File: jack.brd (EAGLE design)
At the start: 44.2 x 26.4 mm, 35 parts, among them IC1 NUF2221W1T2G, IC2 ATSAMD21G18, IC3 LDO, J1 USB-micro, SW1 SPST3.5X6MM, X1 CX-3225 12.288MHz

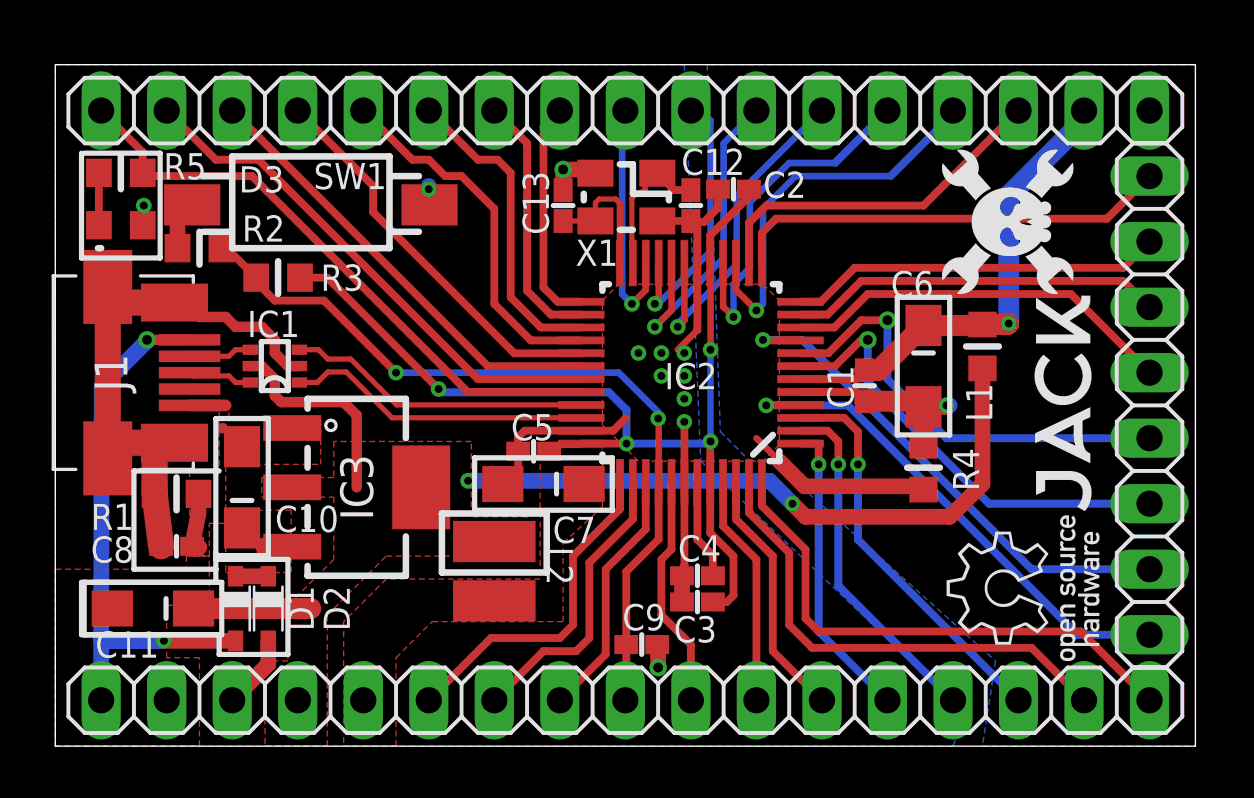
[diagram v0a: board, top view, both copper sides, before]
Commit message: :feelsgood: Added BOM, Gerbers, 3D model and render
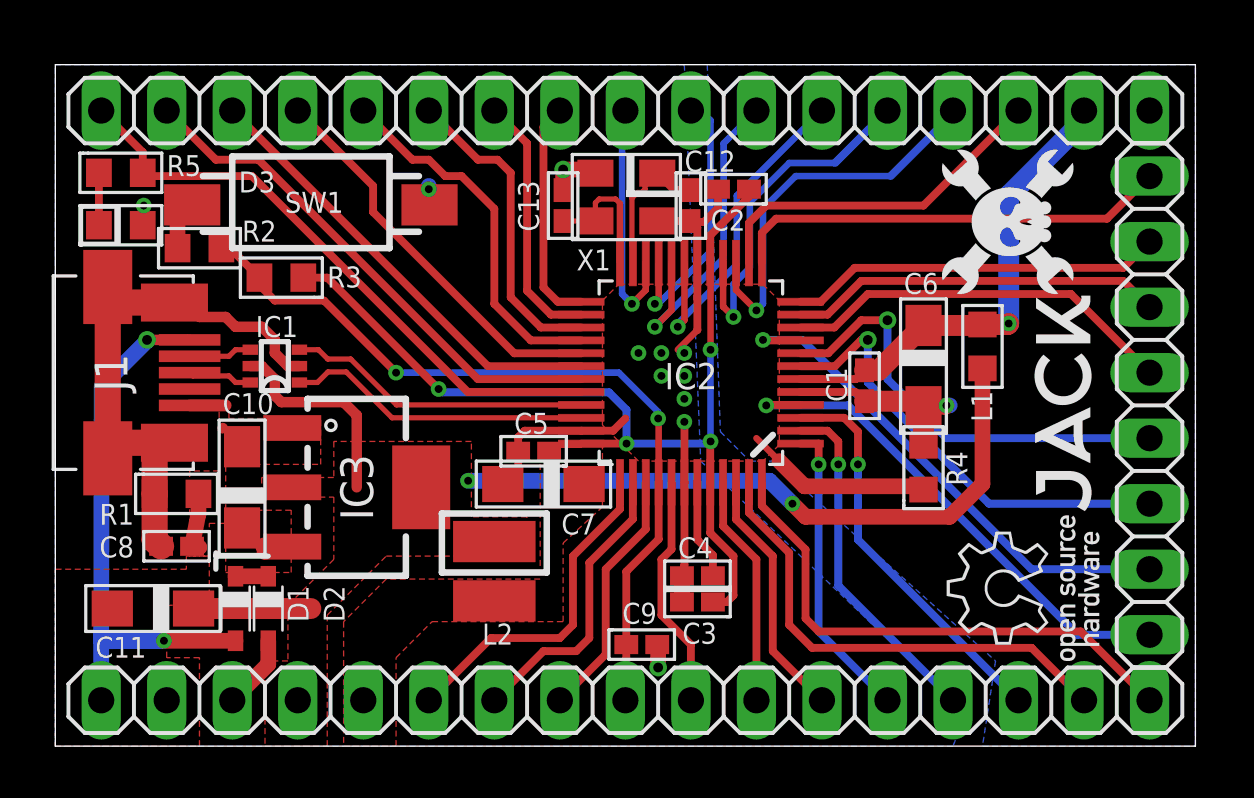
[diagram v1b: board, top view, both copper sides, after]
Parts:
- R5: value 90 -> 68
- moved R3 0.13 mm to (8.76, 18.2)

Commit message: Update of gerber files
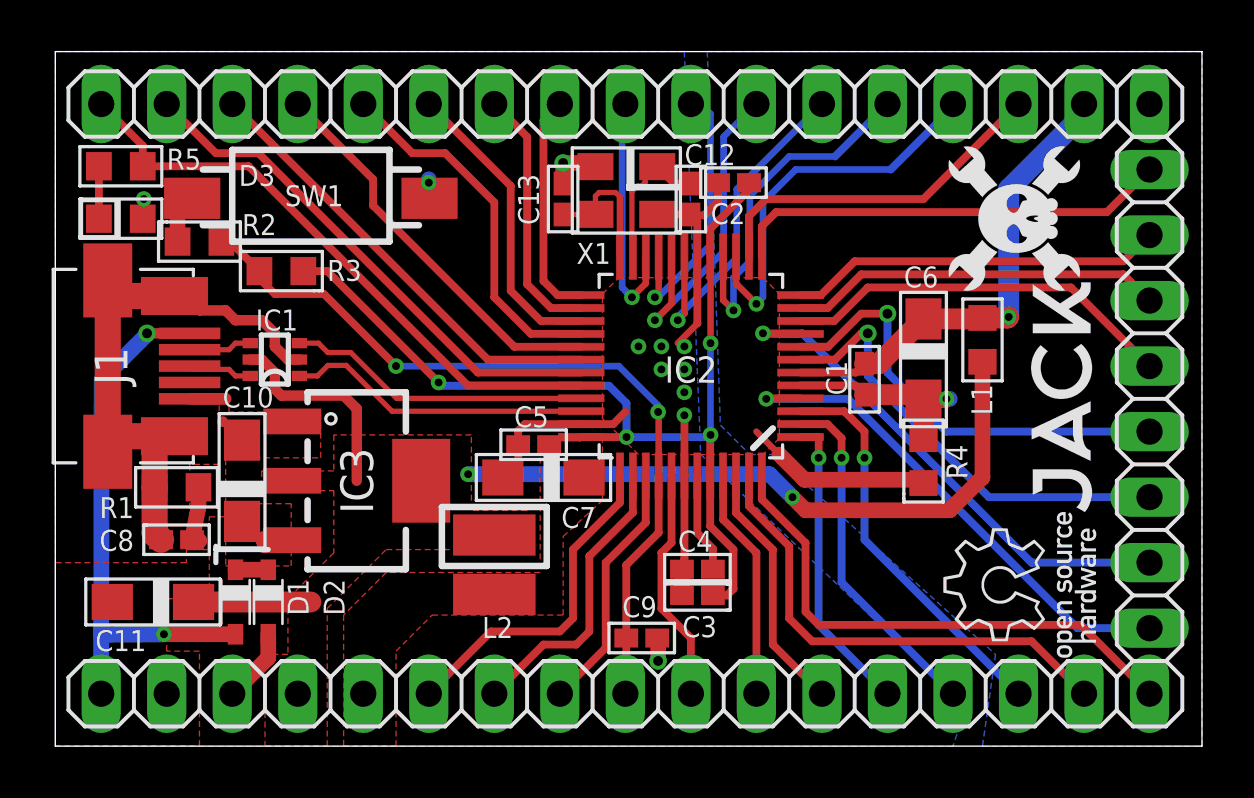
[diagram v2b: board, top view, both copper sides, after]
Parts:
- moved U$5 0.28 mm to (37.6, 20.4)
- moved C10 0.25 mm to (7.24, 10.3)
- moved C12 0.25 mm to (24.6, 21.2)
- moved C13 0.25 mm to (19.7, 21.2)
- moved C2 0.25 mm to (26.3, 21.8)
- moved C6 0.25 mm to (33.7, 15.0)
- moved IC1 0.25 mm to (8.51, 15.0)
- moved IC3 0.25 mm to (11.7, 10.3)
- moved R2 0.25 mm to (5.59, 19.6)
- moved X1 0.25 mm to (22.1, 21.5)
- moved C11 0.25 mm to (3.78, 5.59)
- moved D1 0.25 mm to (6.99, 5.59)
- moved D2 0.25 mm to (8.26, 5.59)
- moved L2 0.25 mm to (17.0, 6.99)
- moved C9 0.25 mm to (22.7, 4.19)
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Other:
- board size 44.2 x 26.4 mm -> 44.5 x 26.9 mm
- board text added: "Copyright © Michele Perla 2015 This documentation describes Open Hardware and is licensed under the CERN OHL v. 1.2. You may redistribute and modify this documentation under the terms of the CERN OHL v.1.2. (http://ohwr.org/cernohl). This documentation is distributed WITHOUT ANY EXPRESS OR IMPLIED WARRANTY, INCLUDING OF MERCHANTABILITY, SATISFACTORY QUALITY AND FITNESS FOR A PARTICULAR PURPOSE. P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"
